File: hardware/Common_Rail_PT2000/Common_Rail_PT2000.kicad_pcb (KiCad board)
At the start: 4 copper layers, 61 x 136.5 mm, 168 parts, among them J1 CONN_01X03, J10 INJ_Term, J11 INJ_Term, J12 INJ_Term, J13 INJ_Term, J15 Conn_01x01, J2 INJ_Term, J4 CONN_02X08, J5 CONN_01X03, J6 CONN_01X03, J8 INJ_Term, J9 INJ_Term, Q1 BUK9230-100B, Q10 BUK9230-100B, Q11 BUK9230-100B, Q12 BUK9230-100B, Q13 BUK9230-100B, Q14 BUK9230-100B, Q15 BUK9230-100B, Q2 BUK9230-100B, Q3 BUK9230-100B, Q4 BUK9230-100B, Q5 BUK9230-100B, Q6 BUK9230-100B, Q7 BUK9230-100B, Q8 BUK9230-100B, Q9 BUK9230-100B, U4 PT2000, Y1 1MHz

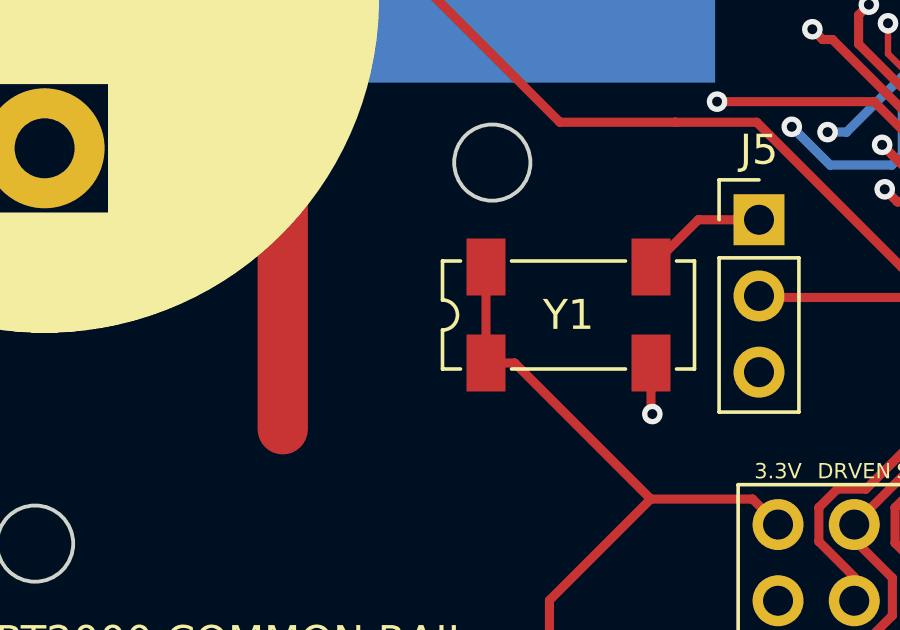
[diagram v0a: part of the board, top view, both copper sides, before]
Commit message: update pcb files
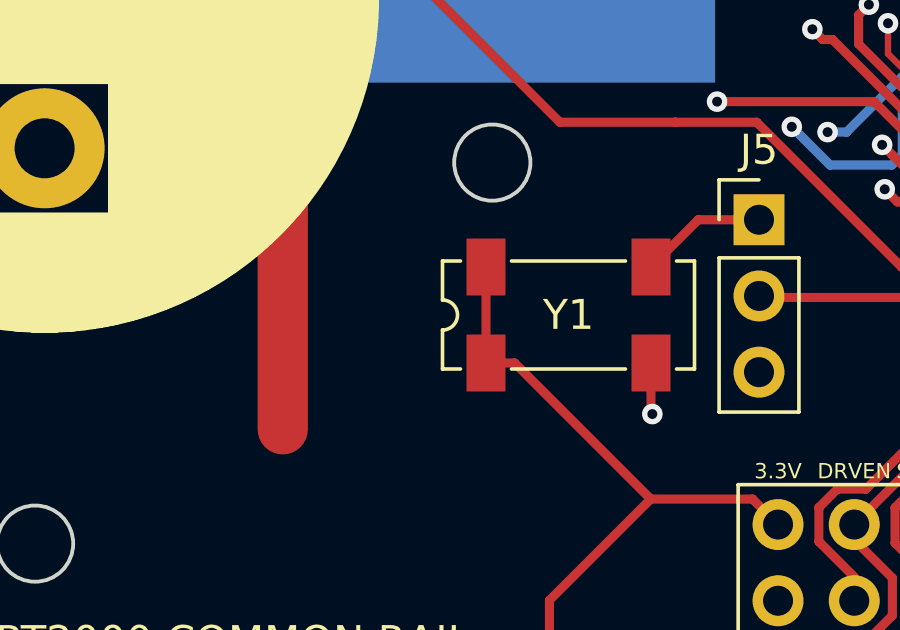
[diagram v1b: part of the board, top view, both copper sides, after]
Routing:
- added copper zone on In1.Cu, net GND
- added copper zone on In2.Cu, net GND
- removed copper zone on GND, net GND
- removed copper zone on PWR_AN, net GND
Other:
- net class 1A external removed
- net class 2.5A external removed
- net class 3.5A external removed
- net class 3.5A external high voltage removed
- net class 5A external removed
- net class Default removed
- net class Supply_200V removed
- net class min2_extern_.188A removed
- net class min_extern_.241A removed
